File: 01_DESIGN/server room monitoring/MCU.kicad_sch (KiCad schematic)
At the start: 10 parts, among them J2 HEADER 4x1, SW1 SW_Push, SW2 SW_Push, U3 ESP32-WROOM-32E

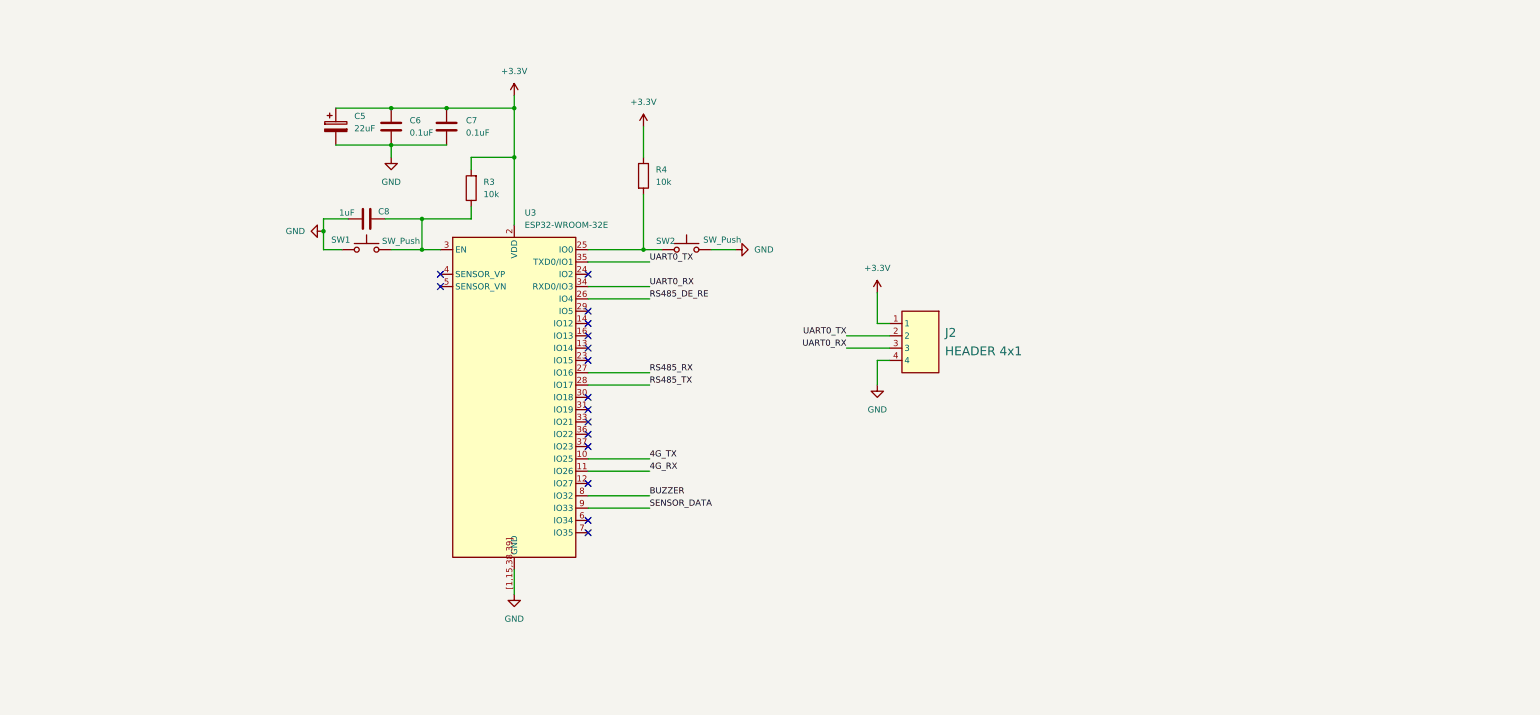
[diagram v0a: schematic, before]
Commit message: Update project files
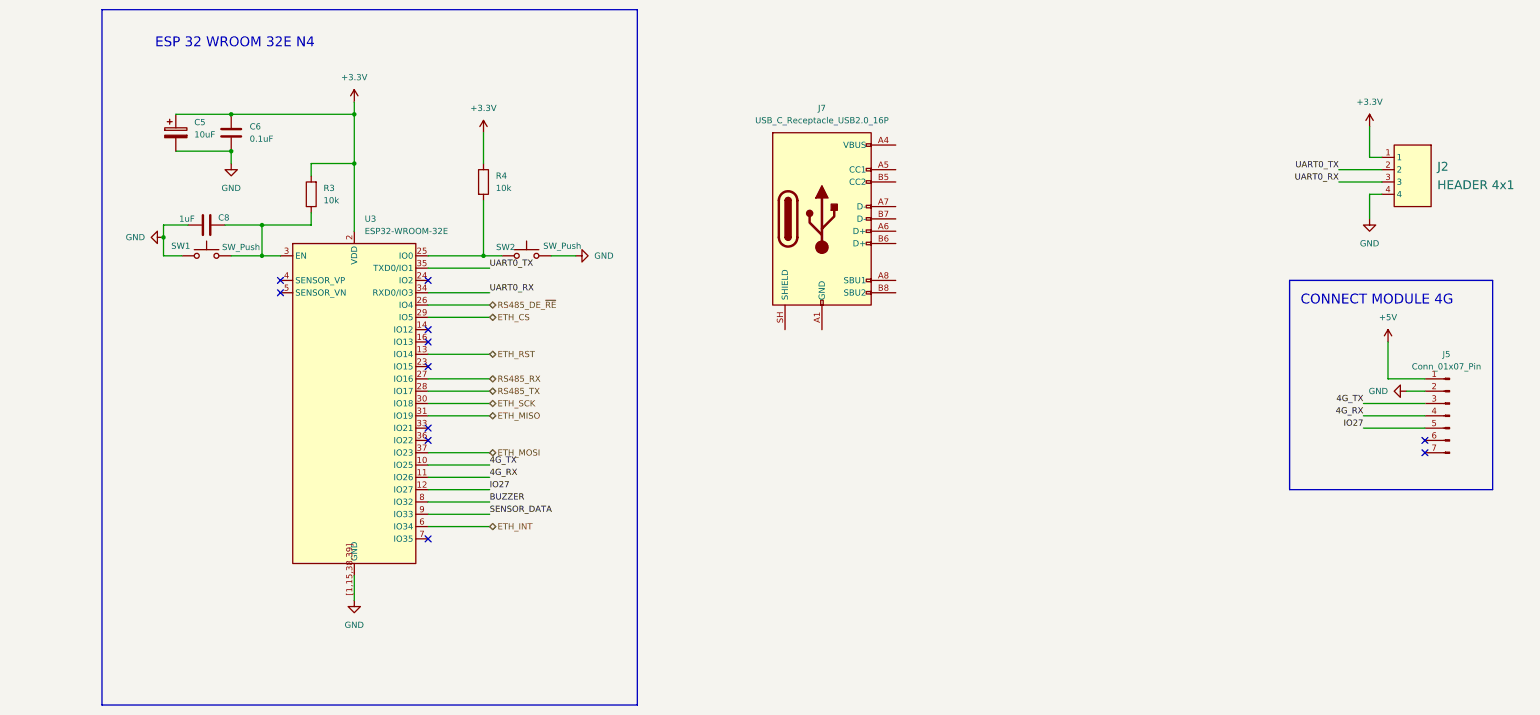
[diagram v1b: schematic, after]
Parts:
- removed C7: 0.1uF, symbol Device:C
- added J5: Conn_01x07_Pin, Connector_PinHeader_2.54mm:PinHeader_1x07_P2.54mm_Vertical, symbol Connector:Conn_01x07_Pin
- added J7: USB_C_Receptacle_USB2.0_16P, Connector_USB:USB3_A_Molex_48393-001, symbol Connector:USB_C_Receptacle_USB2.0_16P
- C5: value 22uF -> 10uF
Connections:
- net 4G_RX: now also J5.4 (Pin_4)
- net 4G_TX: now also J5.3 (Pin_3)
- net GND: now also J5.2 (Pin_2)
- net IO27: now reaches U3.12 (IO27)
- net IO27: now also J5.5 (Pin_5)
- net ETH_RST: now reaches U3.13 (IO14)
- net ETH_CS: now reaches U3.29 (IO5)
- net ETH_SCK: now reaches U3.30 (IO18)
- net ETH_MISO: now reaches U3.31 (IO19)
- net ETH_MOSI: now reaches U3.37 (IO23)
- net ETH_INT: now reaches U3.6 (IO34)
- net RS485_DE_RE renamed RS485_DE_~{RE}
- new net: J7.A1 (GND), J7.A12 (GND), J7.B1 (GND), J7.B12 (GND)
- new net: J7.A4 (VBUS), J7.A9 (VBUS), J7.B4 (VBUS), J7.B9 (VBUS)
- new net +5V: J5.1 (Pin_1)
- no-connect marks 16 -> 11
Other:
- note added: "CONNECT MODULE 4G"
- note added: "ESP 32 WROOM 32E N4"
- moved on the sheet: C5, C6, C8, J2, R3, R4, SW1, SW2, U3

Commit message: Update project files
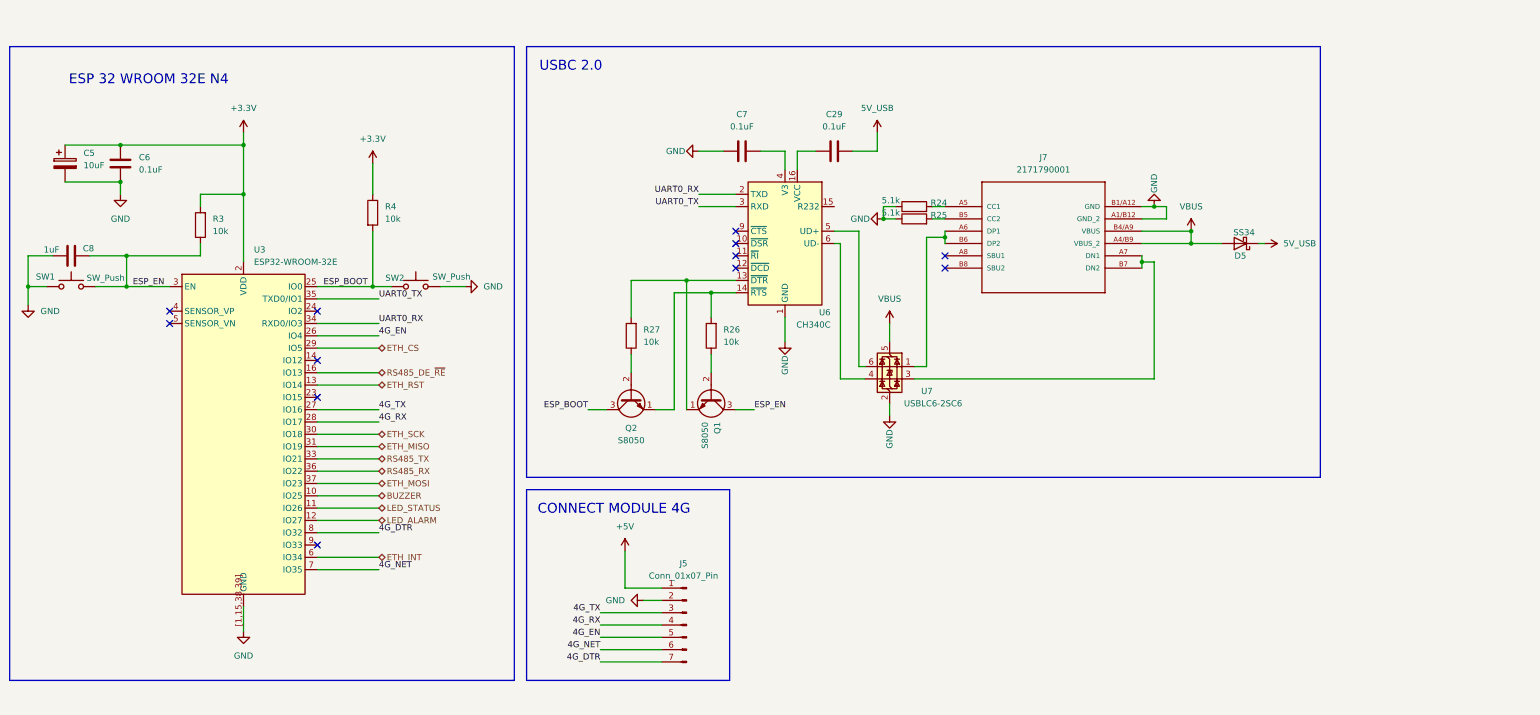
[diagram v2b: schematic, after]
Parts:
- removed J2: HEADER 4x1, symbol AL:Header 4x1
- removed J7: USB_C_Receptacle_USB2.0_16P, Connector_USB:USB3_A_Molex_48393-001, symbol Connector:USB_C_Receptacle_USB2.0_16P
- added C29, C7: 0.1uF, symbol Device:C
- added D5: SS34, Diode_SMD:D_SMA, symbol Diode:SS34
- added J7: 2171790001, 2171790001:2171790001_MOL, symbol 2171790001:2171790001
- added Q1, Q2: S8050, Package_TO_SOT_THT:TO-92_Inline, symbol Transistor_BJT:S8050
- added R24, R25: 5.1k, symbol Device:R
- added R26, R27: 10k, symbol Device:R
- added U6: CH340C, Package_SO:SOIC-16_3.9x9.9mm_P1.27mm, symbol Interface_USB:CH340C
- added U7: USBLC6-2SC6, Package_TO_SOT_SMD:SOT-23-6, symbol Power_Protection:USBLC6-2SC6
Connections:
- net 4G_RX: now also U3.28 (IO17); no longer U3.11 (IO26)
- net 4G_TX: now also U3.27 (IO16); no longer U3.10 (IO25)
- net BUZZER: now also U3.10 (IO25); no longer U3.8 (IO32)
- net GND: now also C7.1, J7.A1/B12 (GND_2), J7.B1/A12 (GND), R24.1, R25.1, U6.1 (GND), U7.2 (GND)
- net RS485_DE_~{RE}: now also U3.16 (IO13); no longer U3.26 (IO4)
- net RS485_RX: now also U3.36 (IO22); no longer U3.27 (IO16)
- net RS485_TX: now also U3.33 (IO21); no longer U3.28 (IO17)
- net UART0_RX: now also U6.2 (TXD)
- net UART0_TX: now also U6.3 (RXD)
- net ESP_EN: now reaches C8.2, R3.1, SW1.2, U3.3 (EN)
- net ESP_EN: now also Q1.3 (C)
- net 4G_NET: now reaches J5.6 (Pin_6)
- net 4G_NET: now also U3.7 (IO35)
- net 4G_DTR: now reaches J5.7 (Pin_7)
- net 4G_DTR: now also U3.8 (IO32)
- net ESP_BOOT: now reaches R4.2, SW2.1, U3.25 (IO0)
- net ESP_BOOT: now also Q2.3 (C)
- net IO27 renamed 4G_EN
- net 4G_EN: now also U3.26 (IO4); no longer U3.12 (IO27)
- net SENSOR_DATA: no longer names the net of U3.9 (IO33)
- new net: Q2.1 (E), R26.2, U6.14 (~{RTS})
- new net: Q2.2 (B), R27.1
- new net: J7.A5 (CC1), R24.2
- new net: Q1.1 (E), R27.2, U6.13 (~{DTR})
- new net: C7.2, U6.4 (V3)
- new net: C29.1, U6.16 (VCC)
- new net: U6.5 (UD+), U7.6 (I/O1)
- new net: U6.6 (UD-), U7.4 (I/O2)
- new net: Q1.2 (B), R26.1
- new net: J7.A6 (DP1), J7.B6 (DP2), U7.1 (I/O1)
- new net: J7.A7 (DN1), J7.B7 (DN2), U7.3 (I/O2)
- new net: J7.B5 (CC2), R25.2
- new net 5V_USB: C29.2, D5.1 (K)
- new net LED_ALARM: U3.12 (IO27)
- new net LED_STATUS: U3.11 (IO26)
- new net VBUS: D5.2 (A), J7.A4/B9 (VBUS_2), J7.B4/A9 (VBUS), U7.5 (VBUS)
- no-connect marks 11 -> 12
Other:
- note added: "USBC 2.0"
- moved on the sheet: C5, C6, C8, J5, R3, R4, SW1, SW2, U3
